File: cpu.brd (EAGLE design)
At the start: 94.2 x 47.8 mm, 86 parts, among them X1 ED060SC4_EINK, X10 PIIKKIRIMA-4, X2 PIIKKIRIMA-5, X3 PIIKKIRIMA-2, X4 629105136821, X5 693071010811, X6 PIIKKIRIMA-6, X7 PIIKKIRIMA-2, X8 PIIKKIRIMA-2, X9 PIIKKIRIMA-2

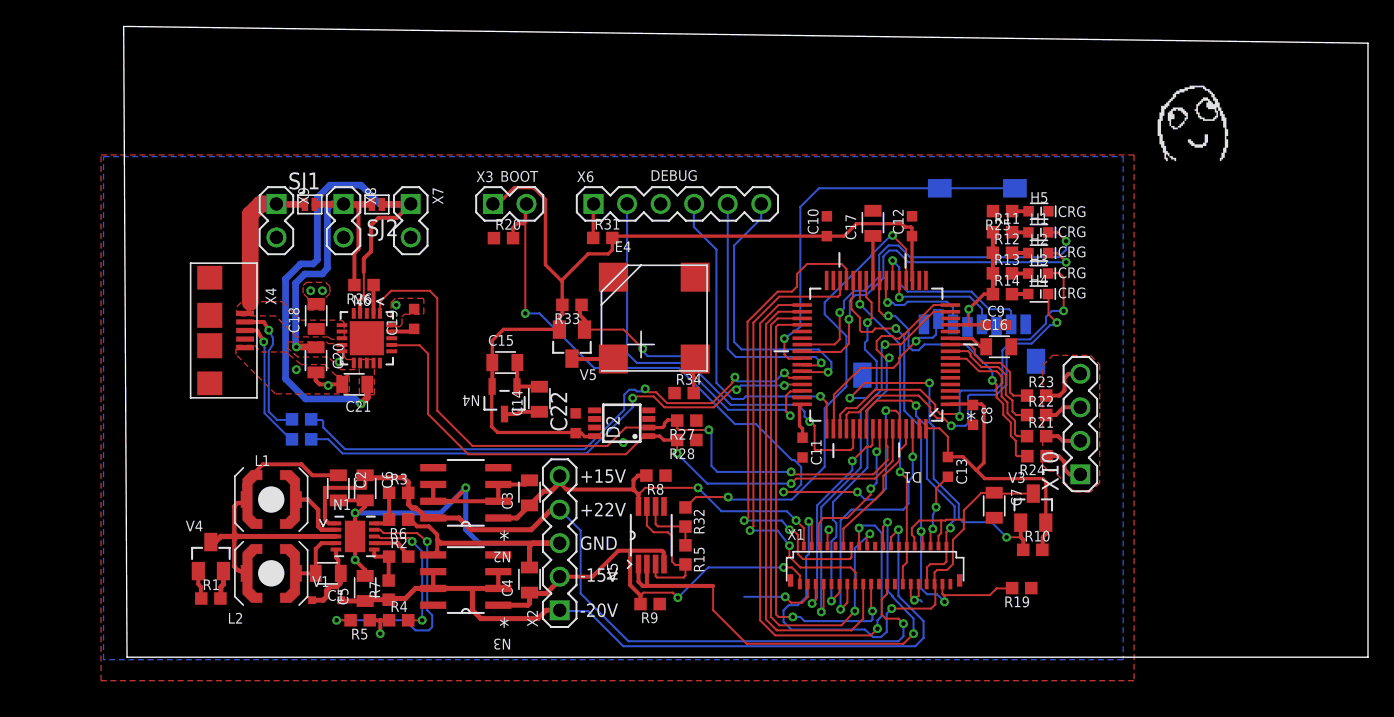
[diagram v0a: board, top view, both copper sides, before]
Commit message: Layout complete
First completed layout , Airwires 0
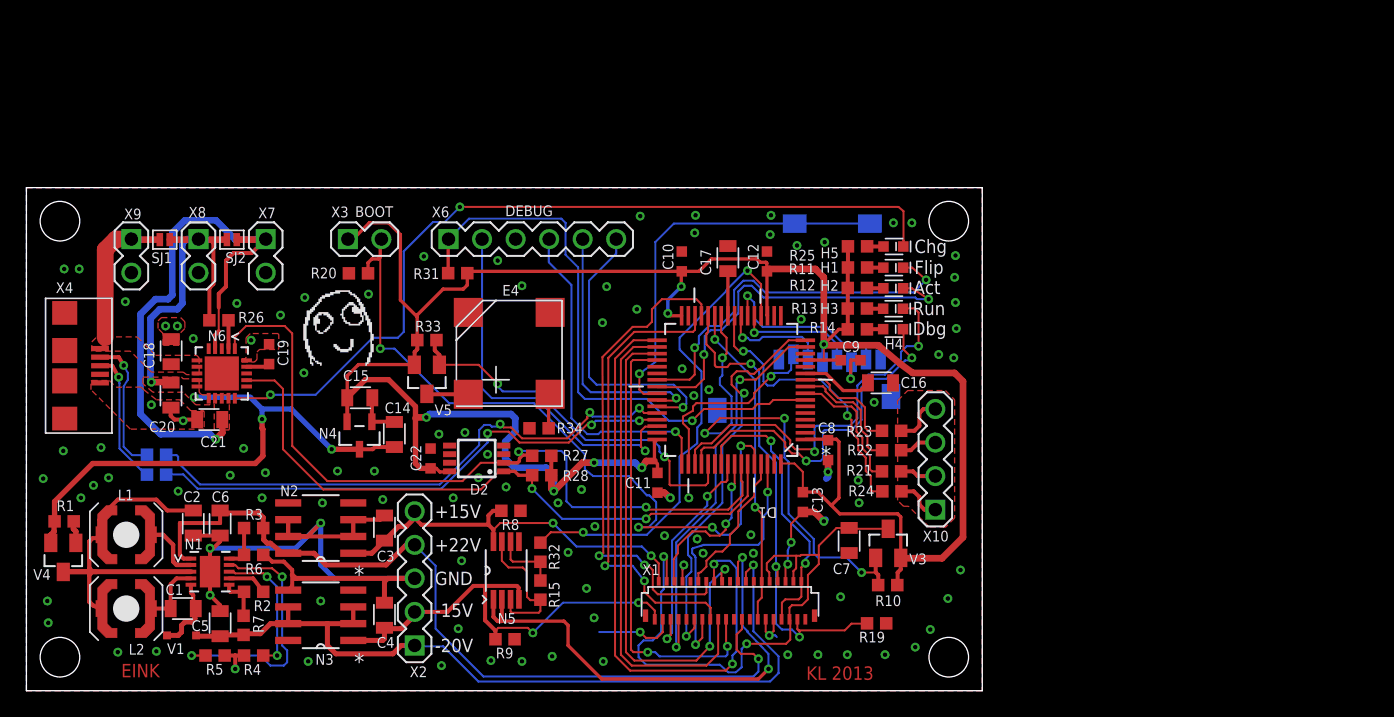
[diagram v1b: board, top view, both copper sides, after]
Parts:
- moved U$2 66.5 mm to (23.8, 27.2)
- moved R1 12.6 mm to (2.86, 12.8), turned to 180 degrees
- moved C12 11.3 mm to (56.1, 32.5)
- moved C7 11.3 mm to (62.3, 11.4)
- moved C9 11.3 mm to (62.4, 25.0)
- moved C10 11.3 mm to (49.6, 32.5)
- moved C13 11.3 mm to (58.8, 14.3)
- moved C15 11.3 mm to (25.2, 22.2)
- moved C17 11.3 mm to (53.1, 32.7)
- moved C19 11.3 mm to (18.4, 25.5)
- moved C22 11.3 mm to (30.6, 17.6)
- moved C3 11.3 mm to (27.1, 12.3)
- moved C4 11.3 mm to (27.1, 5.71)
- moved C8 11.3 mm to (60.7, 18.2)
- moved D1 11.3 mm to (53.4, 22.8)
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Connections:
- net +3V3: now also R25.2
- net VSYS: no longer R25.2
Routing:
- net +3V3: track 108.2 -> 184.0 mm, vias 1 -> 7
- net N$20: track 0.00 -> 63.2 mm, vias 0 -> 2
- net RESETN: track 2.59 -> 44.2 mm, vias 0 -> 1
- net VSYS: track 31.6 -> 67.6 mm, vias 2 -> 4
- net GND: track 84.5 -> 92.9 mm, vias 15 -> 110
- net G8IO4: track 2.98 -> 5.52 mm
- net SCL: track 56.8 -> 58.6 mm
- net NSS1: track 13.7 -> 15.0 mm
- net LED2: track 28.0 -> 29.2 mm
- net BOOT0: track 55.3 -> 56.0 mm
- net LE: track 11.9 -> 12.5 mm
- net EINKD1: track 20.4 -> 20.9 mm
- added copper zone on layer 16, net N$12
- removed copper zone on layer 16, net GND
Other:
- board size 94.2 x 47.8 mm -> 72.4 x 38.1 mm
- board text added: "Act"
- board text added: "Chg"
- board text added: "Dbg"
- board text added: "EINK"
- board text added: "Flip"
- board text added: "KL 2013"
- board text added: "Run"
- board text removed: "CRG"
